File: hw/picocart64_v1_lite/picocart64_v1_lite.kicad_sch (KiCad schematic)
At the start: 16 parts, among them J1 USB_C_Receptacle_USB2.0, J2 Conn_01x05, J3 Conn_02x06_Odd_Even, J4 Micro_SD_Card_Det, Q1 BSS84, SW1 BootButton, U3 RP2040_Stamp, U4 N64-Cartridge

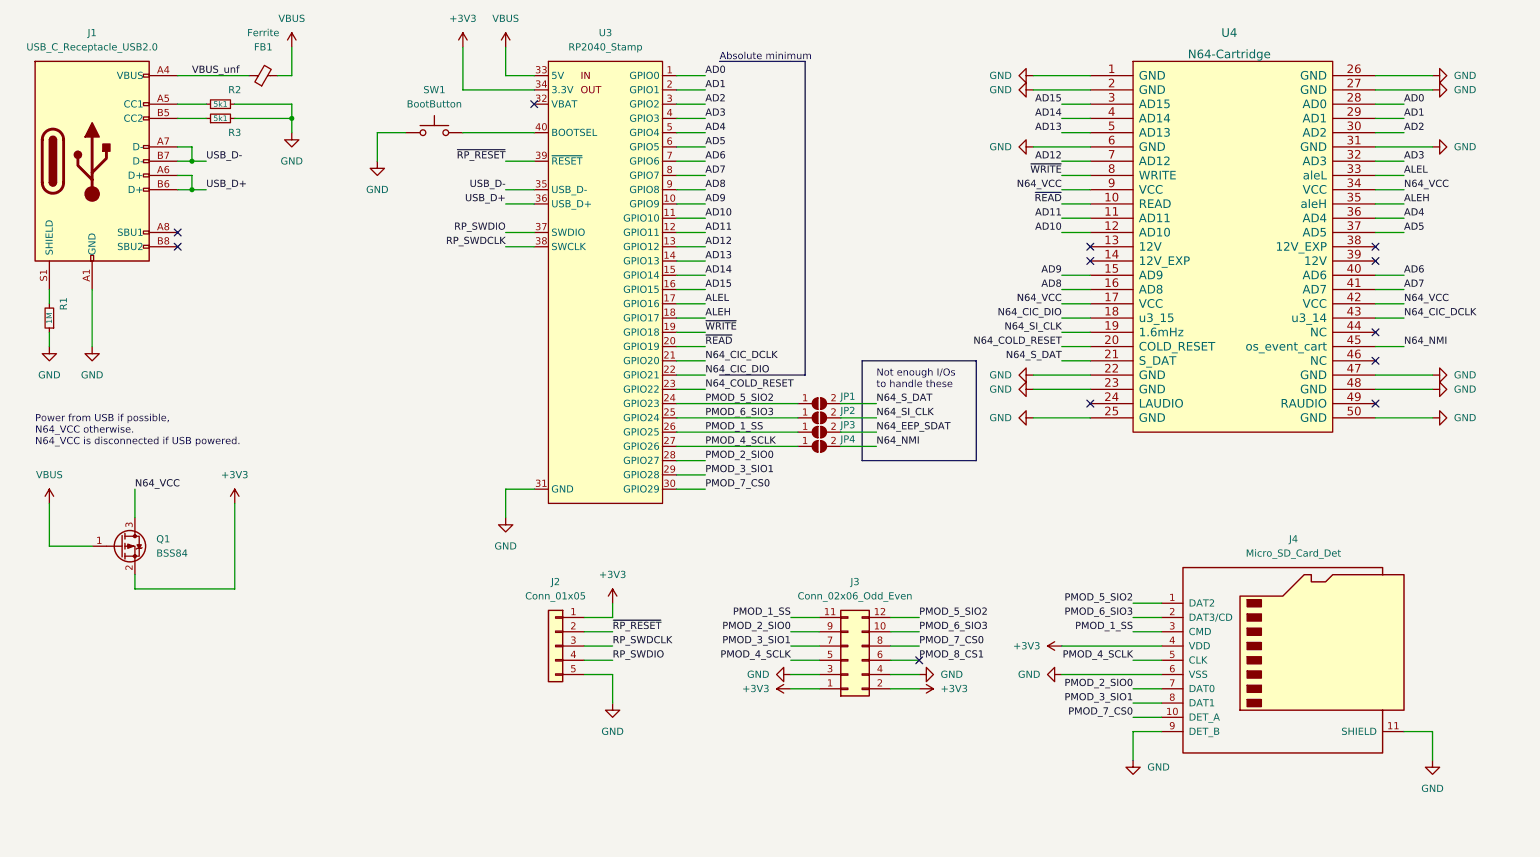
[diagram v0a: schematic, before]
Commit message: hw: Add PicoCart64-lite v1.0
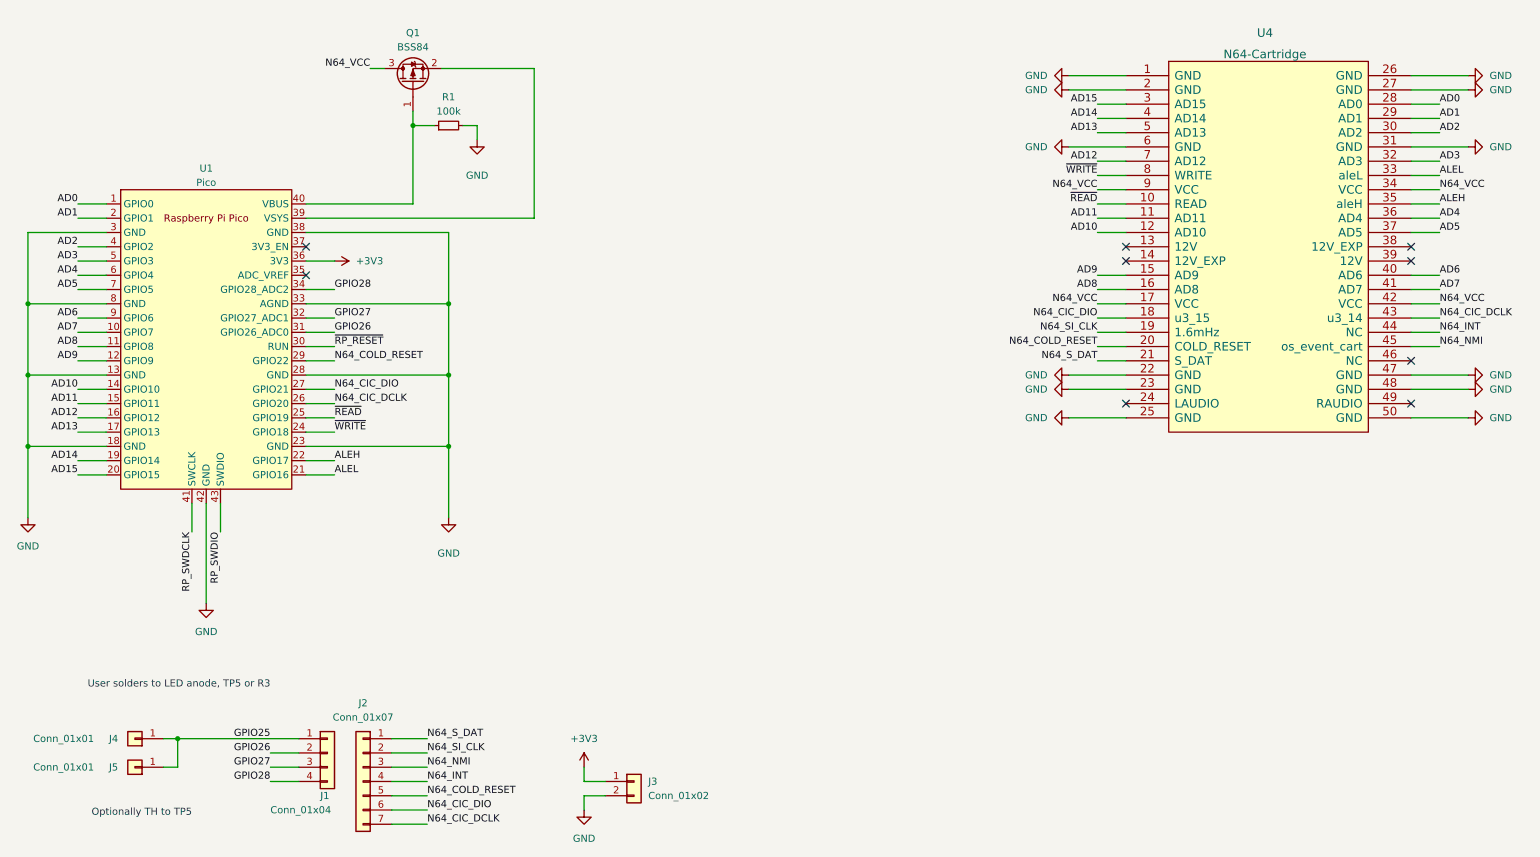
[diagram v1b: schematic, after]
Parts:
- removed FB1: Ferrite, Inductor_SMD:L_0603_1608Metric, symbol Device:FerriteBead_Small
- removed J1: USB_C_Receptacle_USB2.0, Connector_USB_Extra:USB_C_Receptacle_GT-USB-7010, symbol Connector:USB_C_Receptacle_USB2.0
- removed J2: Conn_01x05, Connector_PinHeader_2.54mm:PinHeader_1x05_P2.54mm_Vertical, symbol Connector_Generic:Conn_01x05
- removed J3: Conn_02x06_Odd_Even, Connector_PinSocket_2.54mm:PinSocket_2x06_P2.54mm_Horizontal, symbol Connector_Generic:Conn_02x06_Odd_Even
- removed J4: Micro_SD_Card_Det, Connector_Card:microSD_HC_Molex_104031-0811, symbol Connector:Micro_SD_Card_Det
- removed JP1, JP2, JP3, JP4: SolderJumper_2_Open, Jumper:SolderJumper-2_P1.3mm_Open_TrianglePad1.0x1.5mm, symbol Jumper:SolderJumper_2_Open
- removed R2, R3: 5k1, Resistor_SMD:R_0603_1608Metric, symbol Device:R_Small
- removed SW1: BootButton, Button_Switch_SMD:SW_SPST_FSMSM, symbol Switch:SW_Push
- removed U3: RP2040_Stamp, RP2040_Stamp:RP2040_Stamp_FlexyPin, symbol RP2040_Stamp:RP2040_Stamp
- added J1: Conn_01x04, Connector_PinHeader_2.54mm:PinHeader_1x04_P2.54mm_Vertical, symbol Connector_Generic:Conn_01x04
- added J2: Conn_01x07, Connector_PinHeader_2.54mm:PinHeader_1x07_P2.54mm_Vertical, symbol Connector_Generic:Conn_01x07
- added J3: Conn_01x02, project_area:PinHeader_1x08_P2.54mm_Vertical, symbol Connector_Generic:Conn_01x02
- added J4, J5: Conn_01x01, Connector_PinHeader_2.54mm:PinHeader_1x01_P2.54mm_Vertical, symbol Connector_Generic:Conn_01x01
- added U1: Pico, RPi_Pico:RPi_Pico_SMD_TH, symbol raspberrypi_pico:Pico
- R1: value 1M -> 100k; footprint Resistor_SMD:R_0603_1608Metric -> Resistor_SMD:R_0603_1608Metric_Pad0.98x0.95mm_HandSolder
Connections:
- net +3V3: now also J3.1 (Pin_1), U1.36 (3V3); no longer Q1.2 (S)
- net AD0: now also U1.1 (GPIO0)
- net AD1: now also U1.2 (GPIO1)
- net AD10: now also U1.14 (GPIO10)
- net AD11: now also U1.15 (GPIO11)
- net AD12: now also U1.16 (GPIO12)
- net AD13: now also U1.17 (GPIO13)
- net AD14: now also U1.19 (GPIO14)
- net AD15: now also U1.20 (GPIO15)
- net AD2: now also U1.4 (GPIO2)
- net AD3: now also U1.5 (GPIO3)
- net AD4: now also U1.6 (GPIO4)
- net AD5: now also U1.7 (GPIO5)
- net AD6: now also U1.9 (GPIO6)
- net AD7: now also U1.10 (GPIO7)
- net AD8: now also U1.11 (GPIO8)
- net AD9: now also U1.12 (GPIO9)
- net ALEH: now also U1.22 (GPIO17)
- net ALEL: now also U1.21 (GPIO16)
- net GND: now also R1.2, J3.2 (Pin_2), U1.13 (GND), U1.18 (GND), U1.23 (GND), U1.28 (GND), U1.3 (GND), U1.33 (AGND), U1.38 (GND), U1.42 (GND), U1.8 (GND); no longer R1.1
- net N64_CIC_DCLK: now also J2.7 (Pin_7), U1.26 (GPIO20)
- net N64_CIC_DIO: now also J2.6 (Pin_6), U1.27 (GPIO21)
- net N64_COLD_RESET: now also J2.5 (Pin_5), U1.29 (GPIO22)
- net N64_NMI: now also J2.3 (Pin_3)
- net N64_SI_CLK: now also J2.2 (Pin_2)
- net N64_S_DAT: now also J2.1 (Pin_1)
- net RP_SWDCLK: now also U1.41 (SWCLK)
- net RP_SWDIO: now also U1.43 (SWDIO)
- net ~{READ}: now also U1.25 (GPIO19)
- net ~{RP_RESET}: now also U1.30 (RUN)
- net ~{WRITE}: now also U1.24 (GPIO18)
- net N64_INT: now reaches U4.44 (NC)
- net N64_INT: now also J2.4 (Pin_4)
- net VBUS: no longer names the net of Q1.1 (G)
- net VBUS: now also R1.1, U1.40 (VBUS)
- new net: Q1.2 (S), U1.39 (VSYS)
- new net GPIO25: J1.1 (Pin_1), J4.1 (Pin_1), J5.1 (Pin_1)
- new net GPIO26: J1.2 (Pin_2), U1.31 (GPIO26_ADC0)
- new net GPIO27: J1.3 (Pin_3), U1.32 (GPIO27_ADC1)
- new net GPIO28: J1.4 (Pin_4), U1.34 (GPIO28_ADC2)
- no-connect marks 12 -> 9
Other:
- note added: "Optionally TH to TP5"
- note added: "User solders to LED anode, TP5 or R3"
- note removed: "Absolute minimum"
- note removed: "Not enough I/Os to handle these"
- note removed: "Power from USB if possible, N64_VCC otherwise. N64_VCC is disconnected if USB powered."
- moved on the sheet: U4
